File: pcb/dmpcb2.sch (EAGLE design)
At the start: 65 parts, among them IC1 7805DT, IC2 L293D, IC4 LM358D, IC5 LM358D, J7 SJ-3523-SMT-TR, Q1 IRF530, Q2 IRF530

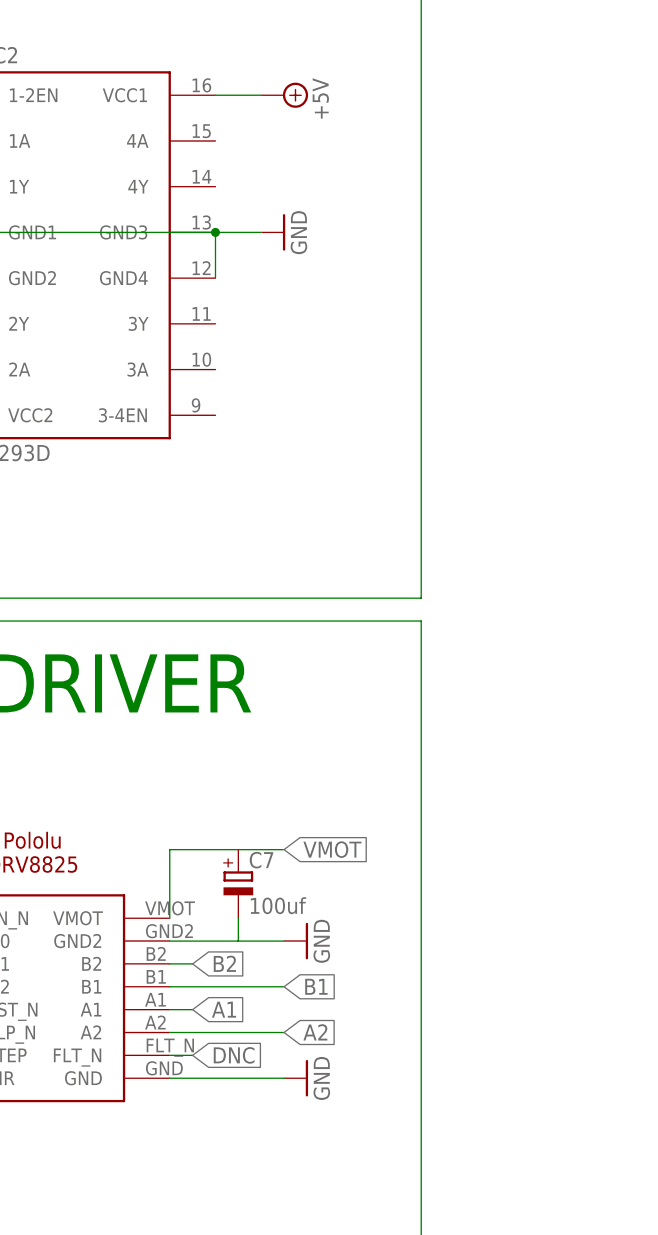
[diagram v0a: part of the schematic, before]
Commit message: borading2..
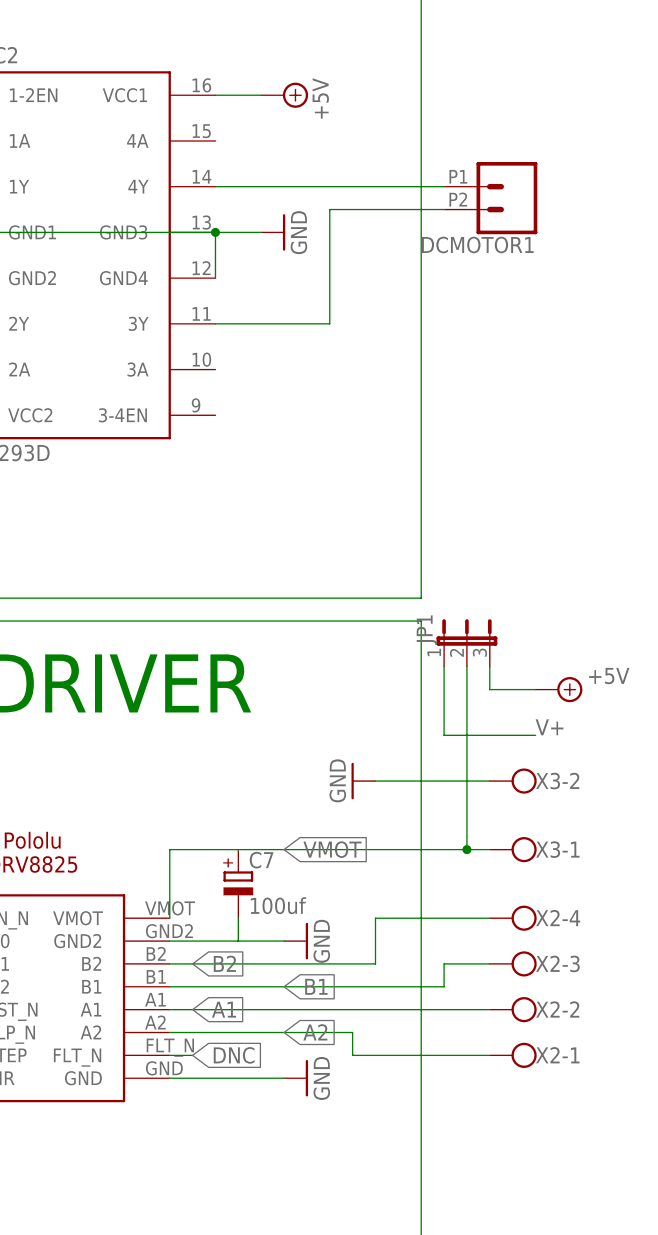
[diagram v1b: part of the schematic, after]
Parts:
- added DCMOTOR1: (no value), SparkFun-Connectors:CONN_022.54MM_SCREWTERM
- added JP1: (no value), jumper:JP2E
- added X2: (no value), con-wago-500:W237-4
- added X3: (no value), con-wago-500:W237-102
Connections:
- new net N$11: DCMOTOR1.1, IC2.4Y
- new net N$12: DCMOTOR1.2, IC2.3Y
- net +5V: now also JP1.3
- net A1: now also X2-2.KL
- net A2: now also X2-1.KL
- net B1: now also X2-3.KL
- net B2: now also X2-4.KL
- net GND: now also X3-2.KL
- net V+: now also JP1.1
- net VMOT: now also JP1.2, X3-1.KL
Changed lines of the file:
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@@
 <part name="D3" library="diode" library_urn="urn:adsk.eagle:library:210" deviceset="1N4148" device="DO35-7" package3d_urn="urn:adsk.eagle:package:43339/2"/>
 <part name="D4" library="diode" library_urn="urn:adsk.eagle:library:210" deviceset="1N4148" device="DO35-7" package3d_urn="urn:adsk.eagle:package:43339/2"/>
+<part name="X2" library="con-wago-500" library_urn="urn:adsk.eagle:library:195" deviceset="W237-4" device="" package3d_urn="urn:adsk.eagle:package:10695/1"/>
+<part name="X3" library="con-wago-500" library_urn="urn:adsk.eagle:library:195" deviceset="W237-102" device="" package3d_urn="urn:adsk.eagle:package:10688/1"/>
+<part name="GND25" library="supply1" library_urn="urn:adsk.eagle:library:371" deviceset="GND" device=""/>
+<part name="JP1" library="jumper" library_urn="urn:adsk.eagle:library:252" deviceset="JP2E" device="" package3d_urn="urn:adsk.eagle:package:15452/1"/>
+<part name="SUPPLY16" library="supply2" library_urn="urn:adsk.eagle:library:372" deviceset="+5V" device=""/>
+<part name="DCMOTOR1" library="SparkFun-Connectors" library_urn="urn:adsk.eagle:library:513" deviceset="CONN_02" device="2.54MM_SCREWTERM" package3d_urn="urn:adsk.eagle:package:38059/1"/>
 </parts>
 <sheets>
@@
 <attribute name="VALUE" x="261.62" y="116.6114" size="1.778" layer="96" rot="R180"/>
 </instance>
+<instance part="X2" gate="-1" x="414.02" y="91.44" smashed="yes" rot="R180">
+<attribute name="NAME" x="414.02" y="90.551" size="1.778" layer="95"/>
+</instance>
+<instance part="X2" gate="-2" x="414.02" y="96.52" smashed="yes" rot="R180">
+<attribute name="NAME" x="414.02" y="95.631" size="1.778" layer="95"/>
+</instance>
+<instance part="X2" gate="-3" x="414.02" y="101.6" smashed="yes" rot="R180">
+<attribute name="NAME" x="414.02" y="100.711" size="1.778" layer="95"/>
+</instance>
+<instance part="X2" gate="-4" x="414.02" y="106.68" smashed="yes" rot="R180">
+<attribute name="VALUE" x="416.56" y="110.363" size="1.778" layer="96" rot="R180"/>
+<attribute name="NAME" x="414.02" y="105.791" size="1.778" layer="95"/>
+</instance>
+<instance part="X3" gate="-1" x="414.02" y="114.3" smashed="yes" rot="R180">
+<attribute name="NAME" x="414.02" y="113.411" size="1.778" layer="95"/>
+</instance>
+<instance part="X3" gate="-2" x="414.02" y="121.92" smashed="yes" rot="R180">
+<attribute name="VALUE" x="416.56" y="125.603" size="1.778" layer="96" rot="R180"/>
+<attribute name="NAME" x="414.02" y="121.031" size="1.778" layer="95"/>
+</instance>
+<instance part="GND25" gate="1" x="393.7" y="121.92" smashed="yes" rot="R270">
+<attribute name="VALUE" x="391.16" y="124.46" size="1.778" layer="96" rot="R270"/>
+</instance>
+<instance part="JP1" gate="1" x="406.4" y="137.16" smashed="yes">
+<attribute name="NAME" x="402.59" y="137.16" size="1.778" layer="95" rot="R90"/>
+<attribute name="VALUE" x="412.115" y="137.16" size="1.778" layer="96" rot="R90"/>
+</instance>
+<instance part="SUPPLY16" gate="+5V" x="416.56" y="132.08" smashed="yes" rot="R270">
+<attribute name="VALUE" x="419.735" y="132.715" size="1.778" layer="96"/>
+</instance>
+<instance part="DCMOTOR1" gate="G$1" x="411.48" y="187.96" smashed="yes" rot="R180">
+<attribute name="VALUE" x="414.02" y="192.786" size="1.778" layer="96" font="vector" rot="R180"/>
+<attribute name="NAME" x="414.02" y="182.372" size="1.778" layer="95" font="vector" rot="R180"/>
+</instance>
 </instances>
 <busses>
@@
 <junction x="297.18" y="114.3"/>
 </segment>
+<segment>
+<pinref part="X3" gate="-2" pin="KL"/>
+<wire x1="408.94" y1="121.92" x2="396.24" y2="121.92" width="0.1524" layer="91"/>
+<pinref part="GND25" gate="1" pin="GND"/>
+</segment>
 </net>
 <net name="V+" class="0">
@@
 <wire x1="345.44" y1="154.94" x2="345.44" y2="162.56" width="0.1524" layer="91"/>
 <wire x1="345.44" y1="162.56" x2="347.98" y2="162.56" width="0.1524" layer="91"/>
+</segment>
+<segment>
+<pinref part="JP1" gate="1" pin="1"/>
+<wire x1="403.86" y1="134.62" x2="403.86" y2="127" width="0.1524" layer="91"/>
+<wire x1="403.86" y1="127" x2="414.02" y2="127" width="0.1524" layer="91"/>
+<label x="414.02" y="127" size="1.778" layer="95"/>
 </segment>
 </net>
@@
 <wire x1="114.3" y1="129.54" x2="114.3" y2="121.92" width="0.1524" layer="91"/>
 </segment>
+<segment>
+<pinref part="JP1" gate="1" pin="3"/>
+<wire x1="408.94" y1="134.62" x2="408.94" y2="132.08" width="0.1524" layer="91"/>
+<wire x1="408.94" y1="132.08" x2="414.02" y2="132.08" width="0.1524" layer="91"/>
+<pinref part="SUPPLY16" gate="+5V" pin="+5V"/>
+</segment>
 </net>
 <net name="N$2" class="0">
@@
 <net name="B2" class="0">
 <segment>
-<wire x1="373.38" y1="101.6" x2="375.92" y2="101.6" width="0.1524" layer="91"/>
 <label x="375.92" y="101.6" size="1.778" layer="95" xref="yes"/>
 <pinref part="U$2" gate="G$1" pin="B2"/>
+<pinref part="X2" gate="-4" pin="KL"/>
+<wire x1="408.94" y1="106.68" x2="396.24" y2="106.68" width="0.1524" layer="91"/>
+<wire x1="396.24" y1="106.68" x2="396.24" y2="101.6" width="0.1524" layer="91"/>
+<wire x1="396.24" y1="101.6" x2="373.38" y2="101.6" width="0.1524" layer="91"/>
 </segment>
 </net>
@@
 <segment>
 <label x="386.08" y="99.06" size="1.778" layer="95" xref="yes"/>
-<wire x1="373.38" y1="99.06" x2="386.08" y2="99.06" width="0.1524" layer="91"/>
 <pinref part="U$2" gate="G$1" pin="B1"/>
+<wire x1="373.38" y1="99.06" x2="403.86" y2="99.06" width="0.1524" layer="91"/>
+<wire x1="403.86" y1="99.06" x2="403.86" y2="101.6" width="0.1524" layer="91"/>
+<pinref part="X2" gate="-3" pin="KL"/>
+<wire x1="403.86" y1="101.6" x2="408.94" y2="101.6" width="0.1524" layer="91"/>
 </segment>
 </net>
 <net name="A1" class="0">
 <segment>
-<wire x1="373.38" y1="96.52" x2="375.92" y2="96.52" width="0.1524" layer="91"/>
 <label x="375.92" y="96.52" size="1.778" layer="95" xref="yes"/>
 <pinref part="U$2" gate="G$1" pin="A1"/>
+<pinref part="X2" gate="-2" pin="KL"/>
+<wire x1="373.38" y1="96.52" x2="408.94" y2="96.52" width="0.1524" layer="91"/>
 </segment>
 </net>
@@
 <segment>
 <label x="386.08" y="93.98" size="1.778" layer="95" xref="yes"/>
-<wire x1="373.38" y1="93.98" x2="386.08" y2="93.98" width="0.1524" layer="91"/>
+<wire x1="373.38" y1="93.98" x2="393.7" y2="93.98" width="0.1524" layer="91"/>
 <pinref part="U$2" gate="G$1" pin="A2"/>
+<wire x1="393.7" y1="93.98" x2="393.7" y2="91.44" width="0.1524" layer="91"/>
+<pinref part="X2" gate="-1" pin="KL"/>
+<wire x1="393.7" y1="91.44" x2="408.94" y2="91.44" width="0.1524" layer="91"/>
 </segment>
 </net>
@@
 <wire x1="373.38" y1="114.3" x2="381" y2="114.3" width="0.1524" layer="91"/>
 <pinref part="C7" gate="G$1" pin="+"/>
-<wire x1="381" y1="114.3" x2="386.08" y2="114.3" width="0.1524" layer="91"/>
 <label x="386.08" y="114.3" size="1.778" layer="95" xref="yes"/>
+<wire x1="381" y1="114.3" x2="406.4" y2="114.3" width="0.1524" layer="91"/>
+<pinref part="X3" gate="-1" pin="KL"/>
+<wire x1="406.4" y1="114.3" x2="408.94" y2="114.3" width="0.1524" layer="91"/>
+<wire x1="406.4" y1="114.3" x2="406.4" y2="134.62" width="0.1524" layer="91"/>
+<junction x="406.4" y="114.3"/>
+<pinref part="JP1" gate="1" pin="2"/>
 </segment>
 </net>
@@
 </segment>
 </net>
+<net name="N$11" class="0">
+<segment>
+<pinref part="IC2" gate="G$1" pin="4Y"/>
+<pinref part="DCMOTOR1" gate="G$1" pin="1"/>
+<wire x1="378.46" y1="187.96" x2="403.86" y2="187.96" width="0.1524" layer="91"/>
+</segment>
+</net>
+<net name="N$12" class="0">
+<segment>
+<pinref part="DCMOTOR1" gate="G$1" pin="2"/>
+<wire x1="403.86" y1="185.42" x2="391.16" y2="185.42" width="0.1524" layer="91"/>
+<wire x1="391.16" y1="185.42" x2="391.16" y2="172.72" width="0.1524" layer="91"/>
+<pinref part="IC2" gate="G$1" pin="3Y"/>
+<wire x1="391.16" y1="172.72" x2="378.46" y2="172.72" width="0.1524" layer="91"/>
+</segment>
+</net>
